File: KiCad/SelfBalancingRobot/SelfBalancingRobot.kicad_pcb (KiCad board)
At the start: 2 copper layers, 3 parts, among them U1 ESP32_NODEMCU, U2 GY-521

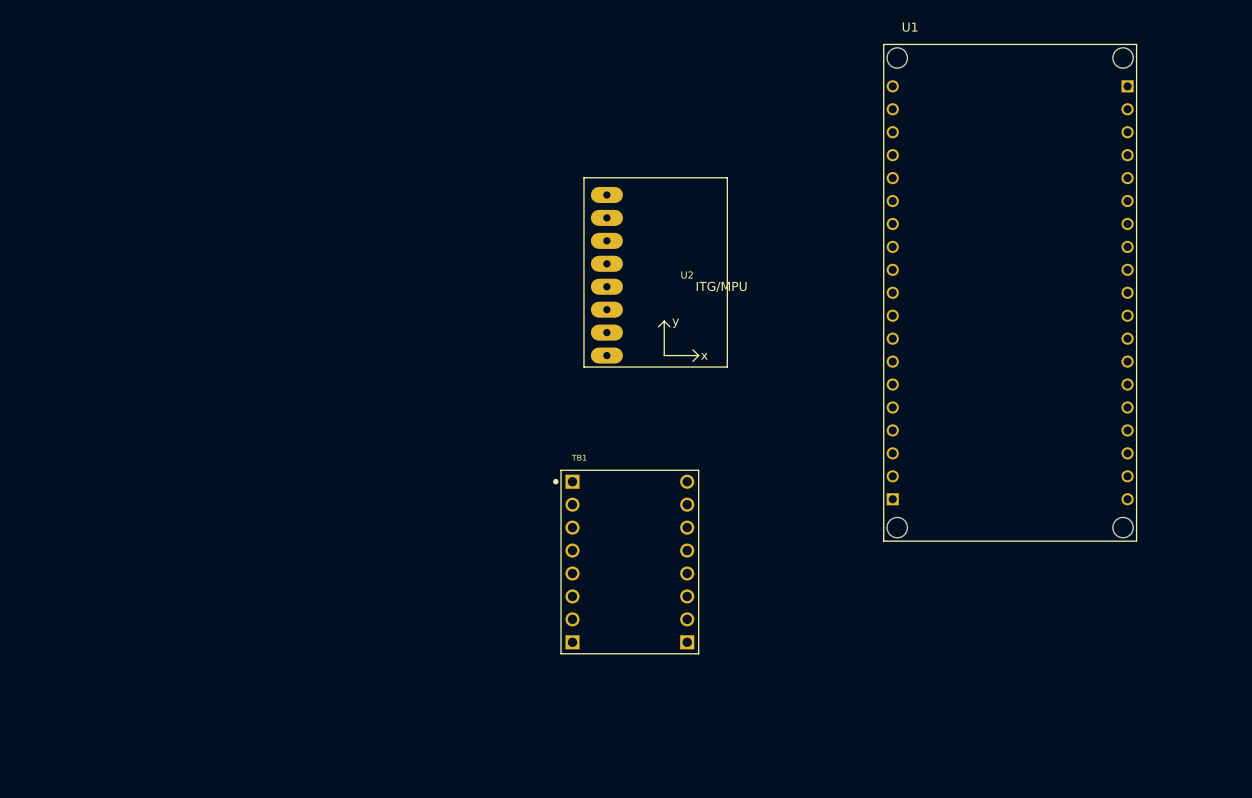
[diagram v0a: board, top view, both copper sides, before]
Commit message: kicad
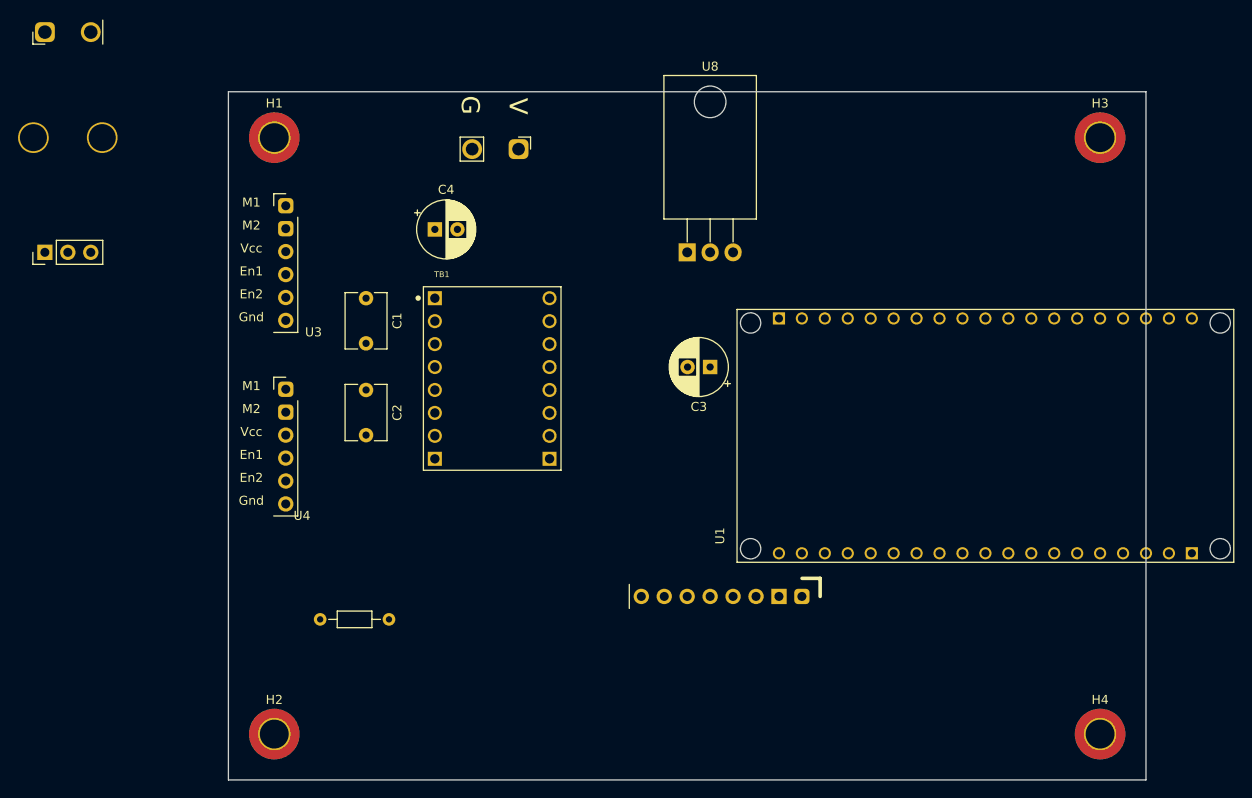
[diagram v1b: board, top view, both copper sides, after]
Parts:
- removed U2: GY-521, 0_Footprints:GY-521
- added C1: C, Capacitor_THT:C_Disc_D6.0mm_W4.4mm_P5.00mm, F.Cu at (116.8, 73.7)
- added C2: C, Capacitor_THT:C_Disc_D6.0mm_W4.4mm_P5.00mm, F.Cu at (116.8, 83.8)
- added C3: C, Capacitor_THT:CP_Radial_D6.3mm_P2.50mm, F.Cu at (154.9, 81.3)
- added C4: C, Capacitor_THT:CP_Radial_D6.3mm_P2.50mm, F.Cu at (124.5, 66.0)
- added H1: MountingHole, MountingHole:MountingHole_3.2mm_M3_DIN965_Pad_TopBottom, F.Cu at (106.7, 55.9)
- added H2: MountingHole, MountingHole:MountingHole_3.2mm_M3_DIN965_Pad_TopBottom, F.Cu at (106.7, 121.9)
- added H3: MountingHole, MountingHole:MountingHole_3.2mm_M3_DIN965_Pad_TopBottom, F.Cu at (198.1, 55.9)
- added H4: MountingHole, MountingHole:MountingHole_3.2mm_M3_DIN965_Pad_TopBottom, F.Cu at (198.1, 121.9)
- added R1: 10kR, Resistor_THT:R_Axial_DIN0204_L3.6mm_D1.6mm_P7.62mm_Horizontal, F.Cu at (119.4, 109.2)
- added U3: ~, 0_Footprints:V-TecMotorHeader, F.Cu at (109.2, 70.1)
- added U4: ~, 0_Footprints:V-TecMotorHeader, F.Cu at (109.2, 90.4)
- added U5: ~, 0_Footprints:BatteryConnector, F.Cu at (127.0, 58.4)
- added U6: ~, 0_Footprints:MPU-6050-External, F.Cu at (147.3, 106.7)
- added U7: ~, 0_Footprints:CurrentMeter, F.Cu at (80.0, 68.6)
- added U8: L7805, Package_TO_SOT_THT:TO-220-3_Horizontal_TabDown, F.Cu at (152.4, 68.6)
- TB1: footprint POLOLU:SHIELD_POLOLU-713 -> 0_Footprints:SHIELD_POLOLU-713
- moved TB1 25.4 mm to (130.8, 82.5)
- moved U1 16.1 mm to (185.4, 88.9), turned to 90 degrees
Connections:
- TB1 pad 1: Net-(TB1-GND-Pad1) -> 0
- TB1 pad 10: unconnected-(TB1-PWMB-Pad10) -> Rmotor-PWM
- TB1 pad 11: unconnected-(TB1-BIN2-Pad11) -> Rmotor-2
- TB1 pad 12: unconnected-(TB1-BIN1-Pad12) -> Rmotor-1
- TB1 pad 13: unconnected-(TB1-~{STBY}-Pad13) -> Net-(TB1-~{STBY})
- TB1 pad 14: unconnected-(TB1-AIN1-Pad14) -> Lmotor-1
- TB1 pad 15: unconnected-(TB1-AIN2-Pad15) -> Lmotor-2
- TB1 pad 16: unconnected-(TB1-PWMA-Pad16) -> Lmotor-PWM
- TB1 pad 2: unconnected-(TB1-VCC-Pad2) -> +3.3V
- TB1 pad 3: unconnected-(TB1-AO1-Pad3) -> Net-(TB1-AO1)
- TB1 pad 4: unconnected-(TB1-AO2-Pad4) -> Net-(TB1-AO2)
- TB1 pad 5: unconnected-(TB1-BO2-Pad5) -> Net-(TB1-BO2)
- TB1 pad 6: unconnected-(TB1-BO1-Pad6) -> Net-(TB1-BO1)
- TB1 pad 7: unconnected-(TB1-VMOT-Pad7) -> +BATT
- TB1 pad 8: Net-(TB1-GND-Pad1) -> 0
- TB1 pad 9: Net-(TB1-GND-Pad1) -> 0
- U1 pad J4_1: unconnected-(U1-GND_J4_1-PadJ4_1) -> 0
- U1 pad J4_10: unconnected-(U1-G5-PadJ4_10) -> Lmotor-PWM
- U1 pad J4_11: unconnected-(U1-G17-PadJ4_11) -> Rmotor-1
- U1 pad J4_12: unconnected-(U1-G16-PadJ4_12) -> Rmotor-2
- U1 pad J4_13: unconnected-(U1-G4-PadJ4_13) -> Rmotor-PWM
- U1 pad J4_15: unconnected-(U1-G2-PadJ4_15) -> LED-Internal
- U1 pad J4_2: unconnected-(U1-G23-PadJ4_2) -> MPU-INT
- U1 pad J4_3: unconnected-(U1-G22-PadJ4_3) -> MPU-SCL
- U1 pad J4_6: unconnected-(U1-G21-PadJ4_6) -> MPU-SDA
- U1 pad J4_7: unconnected-(U1-GND_J4_7-PadJ4_7) -> 0
- U1 pad J4_8: unconnected-(U1-G19-PadJ4_8) -> Lmotor-1
- U1 pad J4_9: unconnected-(U1-G18-PadJ4_9) -> Lmotor-2
- U1 pad J5_1: unconnected-(U1-5V-PadJ5_1) -> +5V
- U1 pad J5_14: unconnected-(U1-G35-PadJ5_14) -> CurrentMeas
- U1 pad J5_16: unconnected-(U1-SN-PadJ5_16) -> RPM-Right
- U1 pad J5_17: unconnected-(U1-SP-PadJ5_17) -> RPM-Left
- U1 pad J5_19: unconnected-(U1-3V3-PadJ5_19) -> +3.3V
- U1 pad J5_6: unconnected-(U1-GND_J5_6-PadJ5_6) -> 0
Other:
- board outline added: 101.6 x 76.2 mm
